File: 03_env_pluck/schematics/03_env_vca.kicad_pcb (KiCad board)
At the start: 2 copper layers, 70 x 75 mm, 69 parts, among them J1 env out 1, J2 gate In 1, J3 signal out, J4 signal in, J5 gate In 2, J6 env out 2, J7 Panel GND, J8 Eurorack, Q1 BC547, Q2 BC547, SW1 Pluck / AD 1, SW2 Pluck / AD 2, U1 LM324, U2 TL072

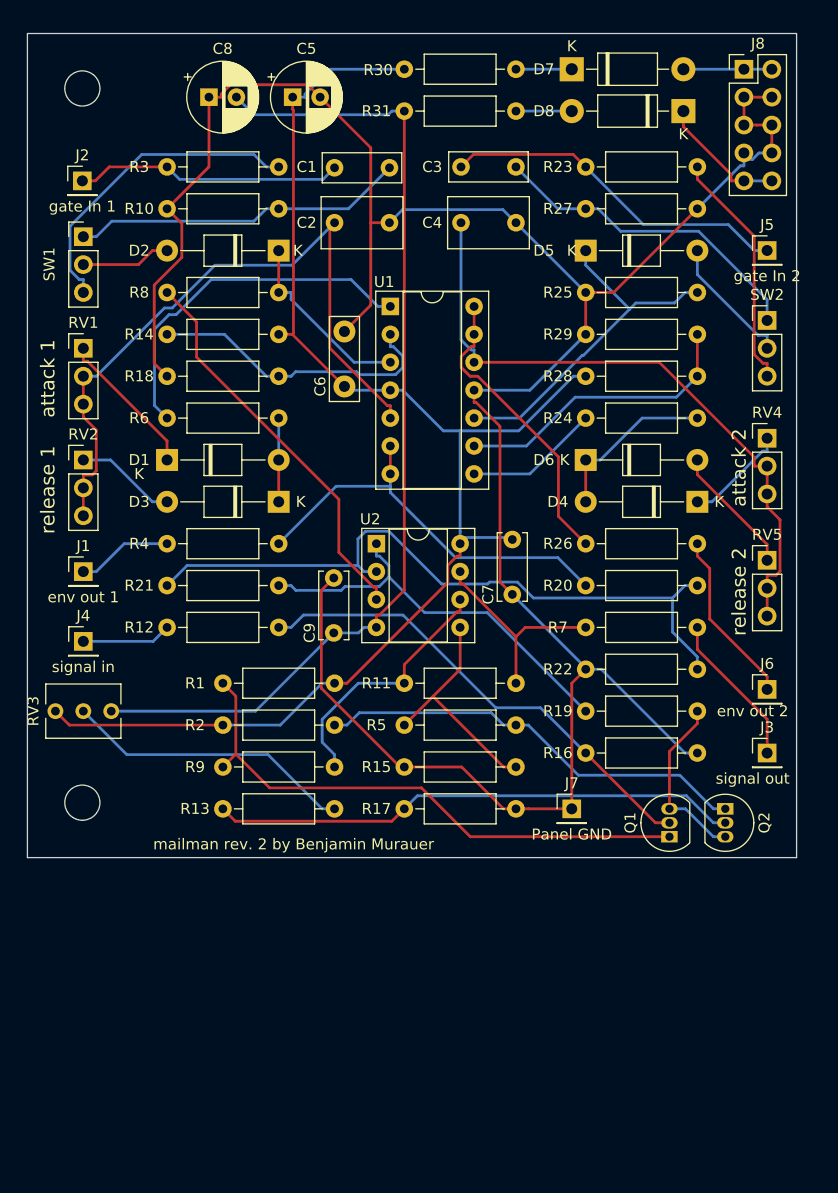
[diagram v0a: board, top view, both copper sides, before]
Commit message: SMD baby
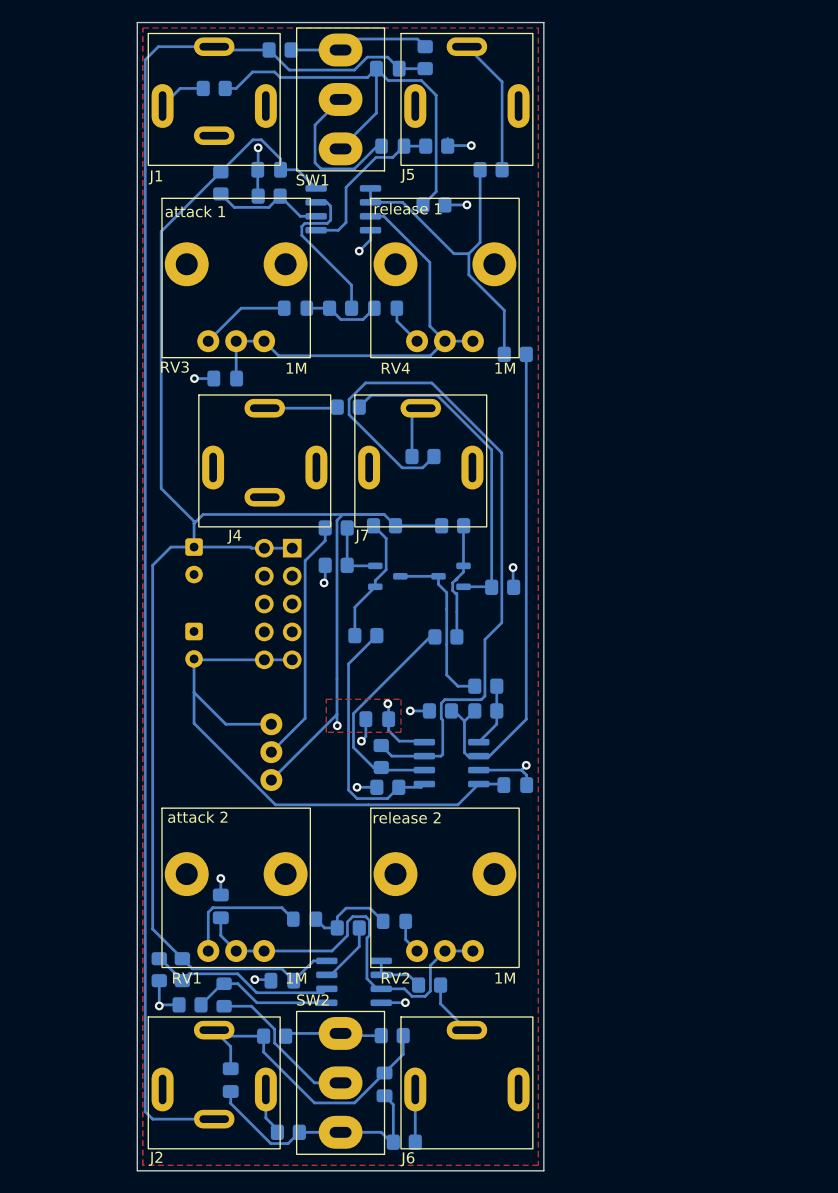
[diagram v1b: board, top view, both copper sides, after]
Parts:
- removed the C3 at (42.5, 15.6)
- removed D7, D8: 1N5819, Diode_THT:D_DO-41_SOD81_P10.16mm_Horizontal
- removed H1, H2: MountingHole, MountingHole:MountingHole_3.2mm_M3
- removed J8: Eurorack, Connector_PinHeader_2.54mm:PinHeader_2x05_P2.54mm_Vertical
- removed the R10 at (15.7, 19.4)
- removed the R23 at (53.8, 15.6)
- removed the R27 at (64.0, 19.4)
- removed the R3 at (15.7, 15.6)
- removed R30, R31: 10, Resistor_THT:R_Axial_DIN0207_L6.3mm_D2.5mm_P10.16mm_Horizontal
- added C10: 100nF, Capacitor_SMD:C_0805_2012Metric_Pad1.18x1.45mm_HandSolder, B.Cu at (47.4, 71.9)
- added C3: 47nF, Capacitor_SMD:C_0805_2012Metric_Pad1.18x1.45mm_HandSolder, B.Cu at (21.5, 98.8)
- added C3: 50uF, Capacitor_THT:CP_Radial_D6.3mm_P2.50mm, B.Cu at (18.2, 50.2)
- added R10: 18k, Resistor_SMD:R_0805_2012Metric_Pad1.20x1.40mm_HandSolder, B.Cu at (25.0, 18.3)
- added R10: 100k, Resistor_SMD:R_0805_2012Metric_Pad1.20x1.40mm_HandSolder, B.Cu at (20.0, 8.50)
- added R23: 100R, Resistor_SMD:R_0805_2012Metric_Pad1.20x1.40mm_HandSolder, B.Cu at (31.1, 51.9)
- added R23: 100k, Resistor_SMD:R_0805_2012Metric_Pad1.20x1.40mm_HandSolder, B.Cu at (25.5, 94.8)
- added R27: 100k, Resistor_SMD:R_0805_2012Metric_Pad1.20x1.40mm_HandSolder, B.Cu at (26.8, 103.5)
- added R27: 100k, Resistor_SMD:R_0805_2012Metric_Pad1.20x1.40mm_HandSolder, B.Cu at (35.2, 69.3)
- added R3: 100k, Resistor_SMD:R_0805_2012Metric_Pad1.20x1.40mm_HandSolder, B.Cu at (26.0, 5.00)
- added R3: 100k, Resistor_SMD:R_0805_2012Metric_Pad1.20x1.40mm_HandSolder, B.Cu at (40.0, 19.1)
- added U3: TL072, Package_SO:SOIC-8_3.9x4.9mm_P1.27mm, B.Cu at (41.6, 69.9)
- C1: footprint Capacitor_THT:C_Rect_L7.0mm_W2.5mm_P5.00mm -> Capacitor_SMD:C_0805_2012Metric_Pad1.18x1.45mm_HandSolder; moved to B.Cu
- C2: value 1uF -> 47nF; footprint Capacitor_THT:C_Rect_L7.2mm_W4.5mm_P5.00mm_FKS2_FKP2_MKS2_MKP2 -> Capacitor_SMD:C_0805_2012Metric_Pad1.18x1.45mm_HandSolder; moved to B.Cu
- C4: value 1uF -> 50uF; footprint Capacitor_THT:C_Rect_L7.2mm_W4.5mm_P5.00mm_FKS2_FKP2_MKS2_MKP2 -> Capacitor_THT:CP_Radial_D6.3mm_P2.50mm; moved to B.Cu
- C5, C8: value 50uF -> 100nF; footprint Capacitor_THT:CP_Radial_D6.3mm_P2.50mm -> Capacitor_SMD:C_0805_2012Metric_Pad1.18x1.45mm_HandSolder; moved to B.Cu
- C6: value 100nF -> 1uF; footprint Capacitor_THT:C_Disc_D7.5mm_W2.5mm_P5.00mm -> Capacitor_SMD:C_0805_2012Metric_Pad1.18x1.45mm_HandSolder; moved to B.Cu
- C7: value 100nF -> 1uF; footprint Capacitor_THT:C_Disc_D6.0mm_W2.5mm_P5.00mm -> Capacitor_SMD:C_0805_2012Metric_Pad1.18x1.45mm_HandSolder; moved to B.Cu
- C9: footprint Capacitor_THT:C_Disc_D6.0mm_W2.5mm_P5.00mm -> Capacitor_SMD:C_0805_2012Metric_Pad1.18x1.45mm_HandSolder; moved to B.Cu
- D1, D2, D3, D4, D5, D6: footprint Diode_THT:D_T-1_P10.16mm_Horizontal -> Diode_SMD:D_0805_2012Metric_Pad1.15x1.40mm_HandSolder; moved to B.Cu
- J1: value env out 1 -> gate in 1; footprint Connector_PinHeader_2.54mm:PinHeader_1x01_P2.54mm_Vertical -> cynthia:3.5mm jack mono switched
- J2: value gate In 1 -> gate in 2; footprint Connector_PinHeader_2.54mm:PinHeader_1x01_P2.54mm_Vertical -> cynthia:3.5mm jack mono switched
- J3: value signal out -> Eurorack; footprint Connector_PinHeader_2.54mm:PinHeader_1x01_P2.54mm_Vertical -> Connector_PinHeader_2.54mm:PinHeader_2x05_P2.54mm_Vertical; moved to B.Cu
- J4: footprint Connector_PinHeader_2.54mm:PinHeader_1x01_P2.54mm_Vertical -> cynthia:3.5mm jack mono switched
- J5: value gate In 2 -> Env out 1; footprint Connector_PinHeader_2.54mm:PinHeader_1x01_P2.54mm_Vertical -> cynthia:3.5mm jack mono
- J6: value env out 2 -> Env out 2; footprint Connector_PinHeader_2.54mm:PinHeader_1x01_P2.54mm_Vertical -> cynthia:3.5mm jack mono
- J7: value Panel GND -> Signal out; footprint Connector_PinHeader_2.54mm:PinHeader_1x01_P2.54mm_Vertical -> cynthia:3.5mm jack mono
- Q1, Q2: footprint Package_TO_SOT_THT:TO-92_Inline -> Package_TO_SOT_SMD:SOT-23-3; moved to B.Cu
- R1, R2: value 20k -> 100k; footprint Resistor_THT:R_Axial_DIN0207_L6.3mm_D2.5mm_P10.16mm_Horizontal -> Resistor_SMD:R_0805_2012Metric_Pad1.20x1.40mm_HandSolder; moved to B.Cu
- R11, R12: value 100k -> 560R; footprint Resistor_THT:R_Axial_DIN0207_L6.3mm_D2.5mm_P10.16mm_Horizontal -> Resistor_SMD:R_0805_2012Metric_Pad1.20x1.40mm_HandSolder; moved to B.Cu
- R13: value 100k -> 1k; footprint Resistor_THT:R_Axial_DIN0207_L6.3mm_D2.5mm_P10.16mm_Horizontal -> Resistor_SMD:R_0805_2012Metric_Pad1.20x1.40mm_HandSolder; moved to B.Cu
- R14: value 82k -> 1k; footprint Resistor_THT:R_Axial_DIN0207_L6.3mm_D2.5mm_P10.16mm_Horizontal -> Resistor_SMD:R_0805_2012Metric_Pad1.20x1.40mm_HandSolder; moved to B.Cu
- R15: footprint Resistor_THT:R_Axial_DIN0207_L6.3mm_D2.5mm_P10.16mm_Horizontal -> Resistor_SMD:R_0805_2012Metric_Pad1.20x1.40mm_HandSolder; moved to B.Cu
- R16, R17: value 100R -> 100k; footprint Resistor_THT:R_Axial_DIN0207_L6.3mm_D2.5mm_P10.16mm_Horizontal -> Resistor_SMD:R_0805_2012Metric_Pad1.20x1.40mm_HandSolder; moved to B.Cu
- R18: value 18k -> 82k; footprint Resistor_THT:R_Axial_DIN0207_L6.3mm_D2.5mm_P10.16mm_Horizontal -> Resistor_SMD:R_0805_2012Metric_Pad1.20x1.40mm_HandSolder; moved to B.Cu
- R19: value 10k -> 100R; footprint Resistor_THT:R_Axial_DIN0207_L6.3mm_D2.5mm_P10.16mm_Horizontal -> Resistor_SMD:R_0805_2012Metric_Pad1.20x1.40mm_HandSolder; moved to B.Cu
- R20, R25: value 100k -> 10k; footprint Resistor_THT:R_Axial_DIN0207_L6.3mm_D2.5mm_P10.16mm_Horizontal -> Resistor_SMD:R_0805_2012Metric_Pad1.20x1.40mm_HandSolder; moved to B.Cu
- R21: value 82k -> 20k; footprint Resistor_THT:R_Axial_DIN0207_L6.3mm_D2.5mm_P10.16mm_Horizontal -> Resistor_SMD:R_0805_2012Metric_Pad1.20x1.40mm_HandSolder; moved to B.Cu
- R22: value 100k -> 20k; footprint Resistor_THT:R_Axial_DIN0207_L6.3mm_D2.5mm_P10.16mm_Horizontal -> Resistor_SMD:R_0805_2012Metric_Pad1.20x1.40mm_HandSolder; moved to B.Cu
- R24, R6: value 560R -> 100k; footprint Resistor_THT:R_Axial_DIN0207_L6.3mm_D2.5mm_P10.16mm_Horizontal -> Resistor_SMD:R_0805_2012Metric_Pad1.20x1.40mm_HandSolder; moved to B.Cu
- R26: value 1k -> 10k; footprint Resistor_THT:R_Axial_DIN0207_L6.3mm_D2.5mm_P10.16mm_Horizontal -> Resistor_SMD:R_0805_2012Metric_Pad1.20x1.40mm_HandSolder; moved to B.Cu
- R28: value 82k -> 100k; footprint Resistor_THT:R_Axial_DIN0207_L6.3mm_D2.5mm_P10.16mm_Horizontal -> Resistor_SMD:R_0805_2012Metric_Pad1.20x1.40mm_HandSolder; moved to B.Cu
- R29: value 18k -> 1k; footprint Resistor_THT:R_Axial_DIN0207_L6.3mm_D2.5mm_P10.16mm_Horizontal -> Resistor_SMD:R_0805_2012Metric_Pad1.20x1.40mm_HandSolder; moved to B.Cu
- R4: value 1k -> 100k; footprint Resistor_THT:R_Axial_DIN0207_L6.3mm_D2.5mm_P10.16mm_Horizontal -> Resistor_SMD:R_0805_2012Metric_Pad1.20x1.40mm_HandSolder; moved to B.Cu
- R5: value 10k -> 100k; footprint Resistor_THT:R_Axial_DIN0207_L6.3mm_D2.5mm_P10.16mm_Horizontal -> Resistor_SMD:R_0805_2012Metric_Pad1.20x1.40mm_HandSolder; moved to B.Cu
- R7: value 1k -> 82k; footprint Resistor_THT:R_Axial_DIN0207_L6.3mm_D2.5mm_P10.16mm_Horizontal -> Resistor_SMD:R_0805_2012Metric_Pad1.20x1.40mm_HandSolder; moved to B.Cu
- R8: value 100k -> 18k; footprint Resistor_THT:R_Axial_DIN0207_L6.3mm_D2.5mm_P10.16mm_Horizontal -> Resistor_SMD:R_0805_2012Metric_Pad1.20x1.40mm_HandSolder; moved to B.Cu
- R9: value 10k -> 82k; footprint Resistor_THT:R_Axial_DIN0207_L6.3mm_D2.5mm_P10.16mm_Horizontal -> Resistor_SMD:R_0805_2012Metric_Pad1.20x1.40mm_HandSolder; moved to B.Cu
- RV1, RV2, RV4: footprint Connector_PinHeader_2.54mm:PinHeader_1x03_P2.54mm_Vertical -> cynthia:potientiometer
- RV3: value 100k -> 1M; footprint Potentiometer_THT:Potentiometer_Vishay_T73XW_Horizontal -> cynthia:potientiometer
- RV5: value 1M -> 100k; footprint Connector_PinHeader_2.54mm:PinHeader_1x03_P2.54mm_Vertical -> cynthia:trimmer; moved to B.Cu
- SW1, SW2: footprint Connector_PinHeader_2.54mm:PinHeader_1x03_P2.54mm_Vertical -> cynthia:switch
- U1: value LM324 -> LM358; footprint Package_DIP:DIP-14_W7.62mm_Socket -> Package_SO:SOIC-8_3.9x4.9mm_P1.27mm; moved to B.Cu
- U2: value TL072 -> LM358; footprint Package_DIP:DIP-8_W7.62mm_Socket -> Package_SO:SOIC-8_3.9x4.9mm_P1.27mm; moved to B.Cu
- moved J2 83.0 mm to (20.0, 99.0)
- moved C5 80.4 mm to (26.2, 89.7), turned to 180 degrees
- moved SW2 79.5 mm to (31.5, 99.0), turned to 180 degrees
- moved C2 78.5 mm to (35.5, 99.1), turned to -90 degrees
- moved R8 61.6 mm to (15.0, 88.7), turned to 90 degrees
- moved U1 61.6 mm to (32.7, 89.8), turned to 180 degrees
- moved R1 59.8 mm to (39.2, 5.70), turned to 90 degrees
- moved R4 55.7 mm to (37.3, 104.4)
- moved R9 53.2 mm to (20.6, 17.1), turned to 90 degrees
- moved RV2 50.0 mm to (41.0, 80.0)
- moved RV1 49.8 mm to (22.0, 80.0)
- moved D1 49.0 mm to (20.9, 91.0), turned to -90 degrees
- moved C6 48.6 mm to (20.6, 82.9)
- moved RV5 48.4 mm to (25.2, 68.9), turned to 90 degrees
- moved R7 48.1 mm to (17.1, 88.7), turned to 90 degrees
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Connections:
- C1 pad 1: Net-(J2-Pin_1) -> Net-(C1-Pad1)
- C2 pad 1: Net-(U1B-+) -> Net-(C2-Pad1)
- C2 pad 2: GND -> Net-(SW2-A)
- C4 pad 1: Net-(U1D-+) -> GND
- C4 pad 2: GND -> -12V
- C6 pad 1: +12V -> Net-(U1A-+)
- C7 pad 1: GND -> Net-(U2A-+)
- C7 pad 2: +12V -> GND
- C8 pad 1: GND -> +12V
- C8 pad 2: -12V -> GND
- C9 pad 1: -12V -> GND
- C9 pad 2: GND -> +12V
- D3 pad 1: Net-(D1-A) -> Net-(D3-K)
- D4 pad 1: Net-(D4-K) -> Net-(D3-A)
- D6 pad 1: Net-(D4-A) -> Net-(D5-A)
- J3 pad 1: Net-(J3-Pin_1) -> +12V
- R1 pad 1: Net-(Q1-C) -> Net-(C1-Pad1)
- R1 pad 2: +12V -> Net-(SW1-C)
- R11 pad 1: Net-(U2B--) -> Net-(R11-Pad1)
- R11 pad 2: Net-(R11-Pad2) -> Net-(D3-A)
- R12 pad 1: Net-(J4-Pin_1) -> Net-(R12-Pad1)
- R12 pad 2: Net-(Q1-B) -> Net-(D5-A)
- R13 pad 1: Net-(Q2-B) -> Net-(U1A--)
- R13 pad 2: Net-(R13-Pad2) -> Net-(J6-PadT)
- R14 pad 1: Net-(U1A--) -> Net-(U2A--)
- R14 pad 2: +12V -> Net-(J5-PadT)
- R15 pad 1: GND -> Net-(U2A--)
- R15 pad 2: Net-(U2B-+) -> Net-(U3A--)
- R16 pad 1: Net-(Q1-B) -> GND
- R16 pad 2: GND -> Net-(U3A--)
- R17 pad 1: Net-(Q2-B) -> Net-(J4-PadT)
- R17 pad 2: GND -> Net-(Q1-B)
- R18 pad 1: GND -> Net-(U3A--)
- R18 pad 2: Net-(U1A--) -> Net-(R18-Pad2)
- R19 pad 1: Net-(R19-Pad1) -> Net-(Q1-B)
- R19 pad 2: Net-(Q1-E) -> GND
- R2 pad 1: +12V -> Net-(C2-Pad1)
- R2 pad 2: Net-(Q2-C) -> Net-(SW2-C)
- R20 pad 1: Net-(U1B--) -> Net-(R18-Pad2)
- R20 pad 2: Net-(U2A--) -> Net-(Q1-E)
- R21 pad 1: Net-(U2A--) -> Net-(Q1-C)
- R21 pad 2: Net-(R19-Pad1) -> +12V
- R22 pad 1: GND -> +12V
- R22 pad 2: Net-(U2A--) -> Net-(Q2-C)
- R24 pad 1: Net-(R24-Pad1) -> Net-(Q2-B)
- R24 pad 2: Net-(D4-A) -> Net-(R24-Pad2)
- R25 pad 1: GND -> Net-(U3B-+)
- R25 pad 2: Net-(D5-K) -> Net-(Q2-C)
- R26 pad 1: Net-(U1D--) -> Net-(Q1-C)
- R26 pad 2: Net-(J6-Pin_1) -> Net-(U3B--)
- R28 pad 1: Net-(U1C--) -> GND
- R28 pad 2: +12V -> Net-(U3B-+)
- R29 pad 1: GND -> Net-(R27-Pad2)
- R29 pad 2: Net-(U1C--) -> Net-(J7-PadT)
- R4 pad 1: Net-(U1B--) -> GND
- R4 pad 2: Net-(J1-Pin_1) -> Net-(SW2-A)
- R5 pad 1: Net-(U2B-+) -> GND
- R5 pad 2: Net-(Q2-C) -> Net-(D1-K)
- R6 pad 1: Net-(R6-Pad1) -> GND
- R6 pad 2: Net-(D1-A) -> Net-(D2-K)
- R7 pad 1: Net-(R11-Pad2) -> Net-(U1B--)
- R7 pad 2: Net-(J3-Pin_1) -> +12V
- R8 pad 1: GNDREF -> GND
- R8 pad 2: Net-(D2-K) -> Net-(U1B--)
- R9 pad 1: Net-(Q1-C) -> Net-(U2B--)
- R9 pad 2: Net-(U2B--) -> +12V
- RV1 pad 1: Net-(D1-K) -> Net-(D3-K)
- RV1 pad 2: Net-(U1B-+) -> Net-(U1A-+)
- RV1 pad 3: Net-(U1B-+) -> Net-(U1A-+)
- RV2 pad 1: Net-(D3-A) -> Net-(D4-A)
- RV2 pad 2: Net-(U1B-+) -> Net-(U1A-+)
- RV2 pad 3: Net-(U1B-+) -> Net-(U1A-+)
- RV3 pad 1: +12V -> Net-(D5-K)
- RV3 pad 2: Net-(R13-Pad2) -> Net-(U2A-+)
- RV3 pad 3: -12V -> Net-(U2A-+)
- RV4 pad 1: Net-(D4-K) -> Net-(D6-A)
- RV4 pad 2: Net-(U1D-+) -> Net-(U2A-+)
- RV4 pad 3: Net-(U1D-+) -> Net-(U2A-+)
- RV5 pad 1: Net-(D6-A) -> +12V
- RV5 pad 2: Net-(U1D-+) -> Net-(R24-Pad2)
- RV5 pad 3: Net-(U1D-+) -> -12V
- SW2 pad 2: Net-(D5-A) -> Net-(D1-A)
- U1 pad 1: Net-(R6-Pad1) -> Net-(U1A--)
- U1 pad 3: Net-(D2-K) -> Net-(U1A-+)
- U1 pad 4: +12V -> GND
- U1 pad 5: Net-(U1B-+) -> Net-(D1-K)
- U1 pad 7: Net-(U1B--) -> Net-(R11-Pad1)
- U1 pad 8: Net-(R24-Pad1) -> +12V
- U2 pad 1: Net-(R19-Pad1) -> Net-(U2A--)
- U2 pad 3: GNDREF -> Net-(U2A-+)
- U2 pad 4: -12V -> GND
- U2 pad 5: Net-(U2B-+) -> Net-(D2-K)
- U2 pad 7: Net-(R11-Pad2) -> Net-(R12-Pad1)
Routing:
- net GND: track 231.2 -> 51.6 mm, vias 0 -> 15
- net Net-(C1-Pad1): track 0.00 -> 130.5 mm
- net Net-(R27-Pad2): track 0.00 -> 66.5 mm
- net Net-(U1B-+): track 63.2 -> 0.00 mm
- net Net-(U1D-+): track 59.5 -> 0.00 mm
- net +12V: track 127.5 -> 176.1 mm, vias 0 -> 2
- net Net-(U3A--): track 0.00 -> 46.1 mm
- net Net-(Q2-B): track 48.2 -> 5.98 mm
- net Net-(U2A-+): track 0.00 -> 41.3 mm
- net Net-(Q1-C): track 51.2 -> 10.8 mm
- net Net-(R19-Pad1): track 37.3 -> 0.00 mm
- net -12V: track 91.6 -> 54.4 mm
- net Net-(U1A-+): track 0.00 -> 36.7 mm
- net GNDREF: track 36.0 -> 0.00 mm
- net Net-(U2A--): track 64.2 -> 30.7 mm
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- added copper zone on F.Cu, net +12V
- added copper zone on F.Cu, net GND
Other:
- board size 70 x 75 mm -> 37 x 104.5 mm
- board text removed: "mailman rev. 2 by Benjamin Murauer"
